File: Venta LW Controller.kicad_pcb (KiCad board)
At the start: 2 copper layers, 56 x 99.2 mm, 29 parts, among them J1 Conn_01x04, J2 Conn_02x05_Odd_Even, Q1 BSS138, Q2 BSS138, SW1 RST, SW2 FLASH, U1 LM2674N-3.3, U2 ESP-12F

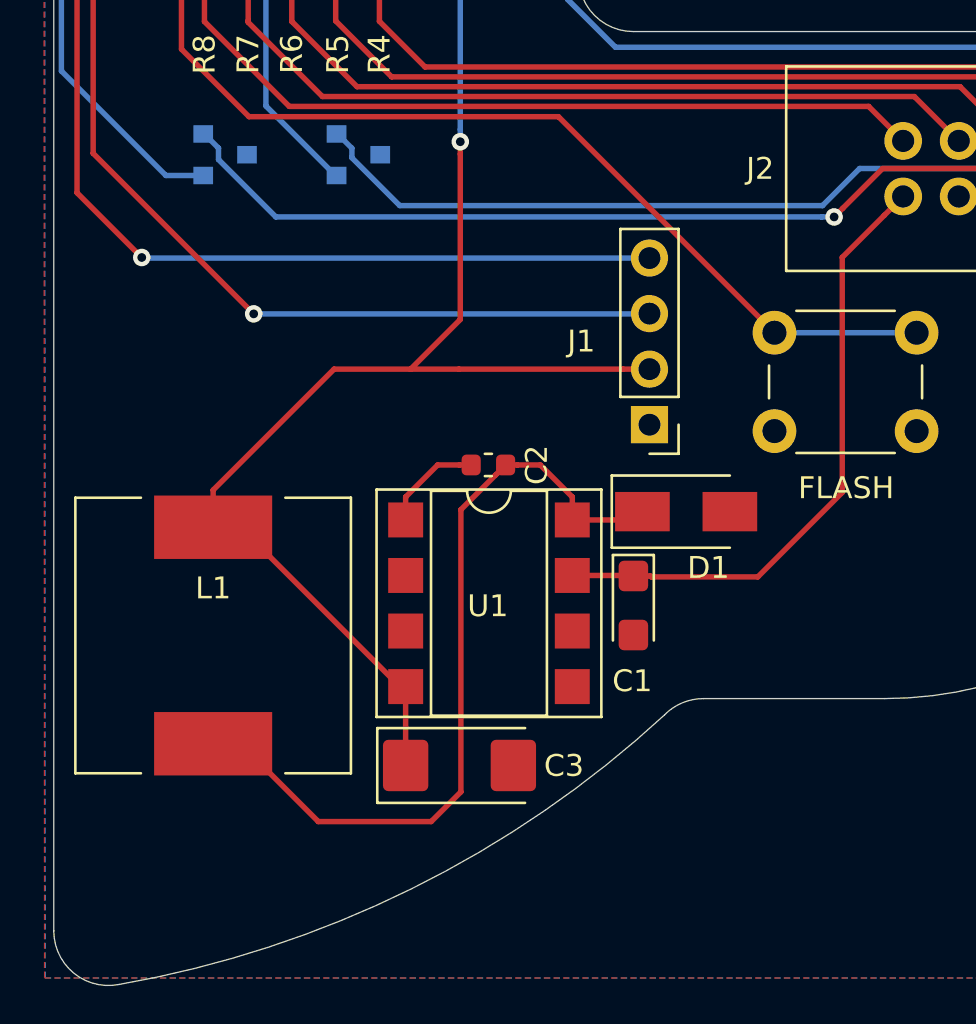
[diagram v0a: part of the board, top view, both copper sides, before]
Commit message: updated package
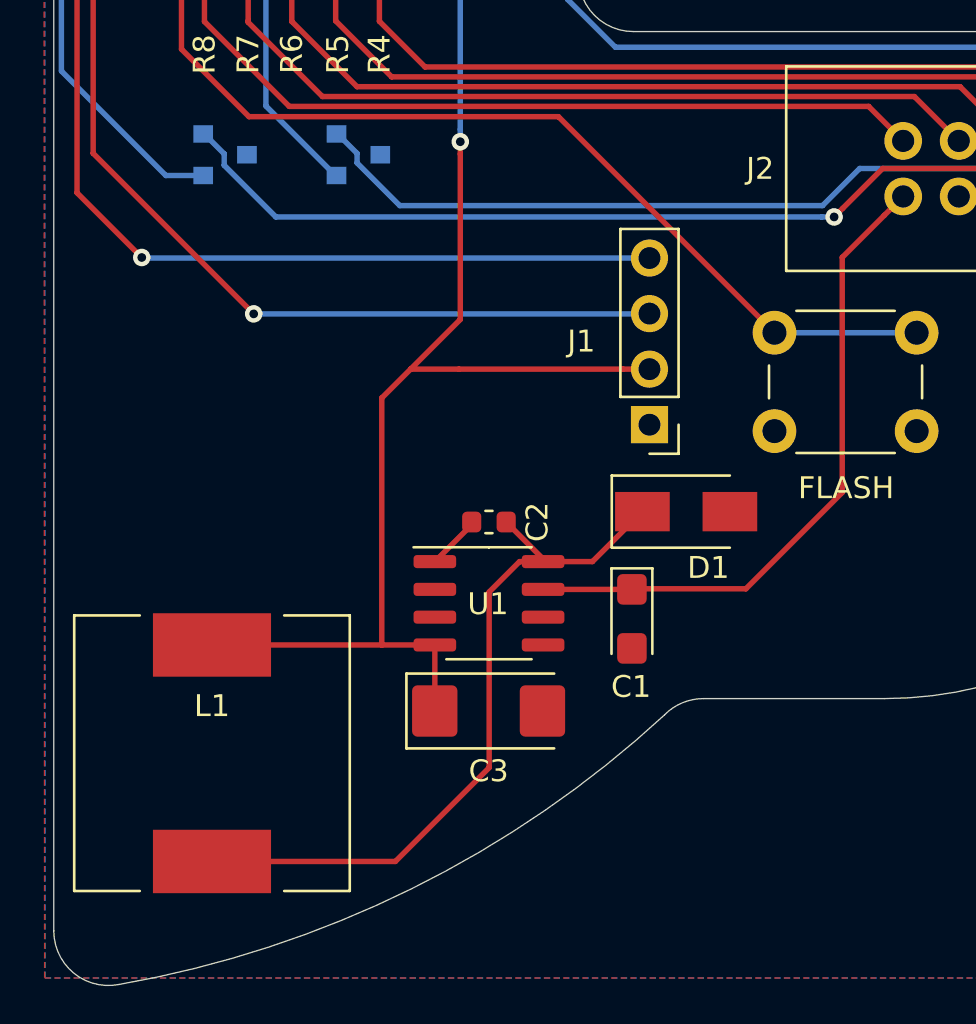
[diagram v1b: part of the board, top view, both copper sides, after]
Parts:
- U1: footprint Package_DIP:DIP-8_W7.62mm_SMDSocket_SmallPads -> Package_SO:SOIC-8_3.9x4.9mm_P1.27mm
- moved L1 5.38 mm to (131.7, 131.0)
- moved C3 2.82 mm to (144.4, 129.1)
- moved C2 2.61 mm to (144.4, 120.4)
- moved C1 0.62 mm to (150.9, 124.9)
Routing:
- net Net-(C2-Pad2): track 37.2 -> 33.5 mm
- net Net-(C2-Pad1): track 4.65 -> 2.51 mm
- net +3.3V: track 84.6 -> 82.5 mm
- net +24V: track 28.7 -> 30.2 mm
